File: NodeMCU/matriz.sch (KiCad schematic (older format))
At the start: 16 parts, among them J1 Conn_01x05, Q1 Q_NPN_CBE, Q2 Q_NPN_CBE, Q3 Q_NPN_CBE, SW1 SW_Push_Open, SW2 SW_Push, U3 NodeMCU1.0(ESP-12E)

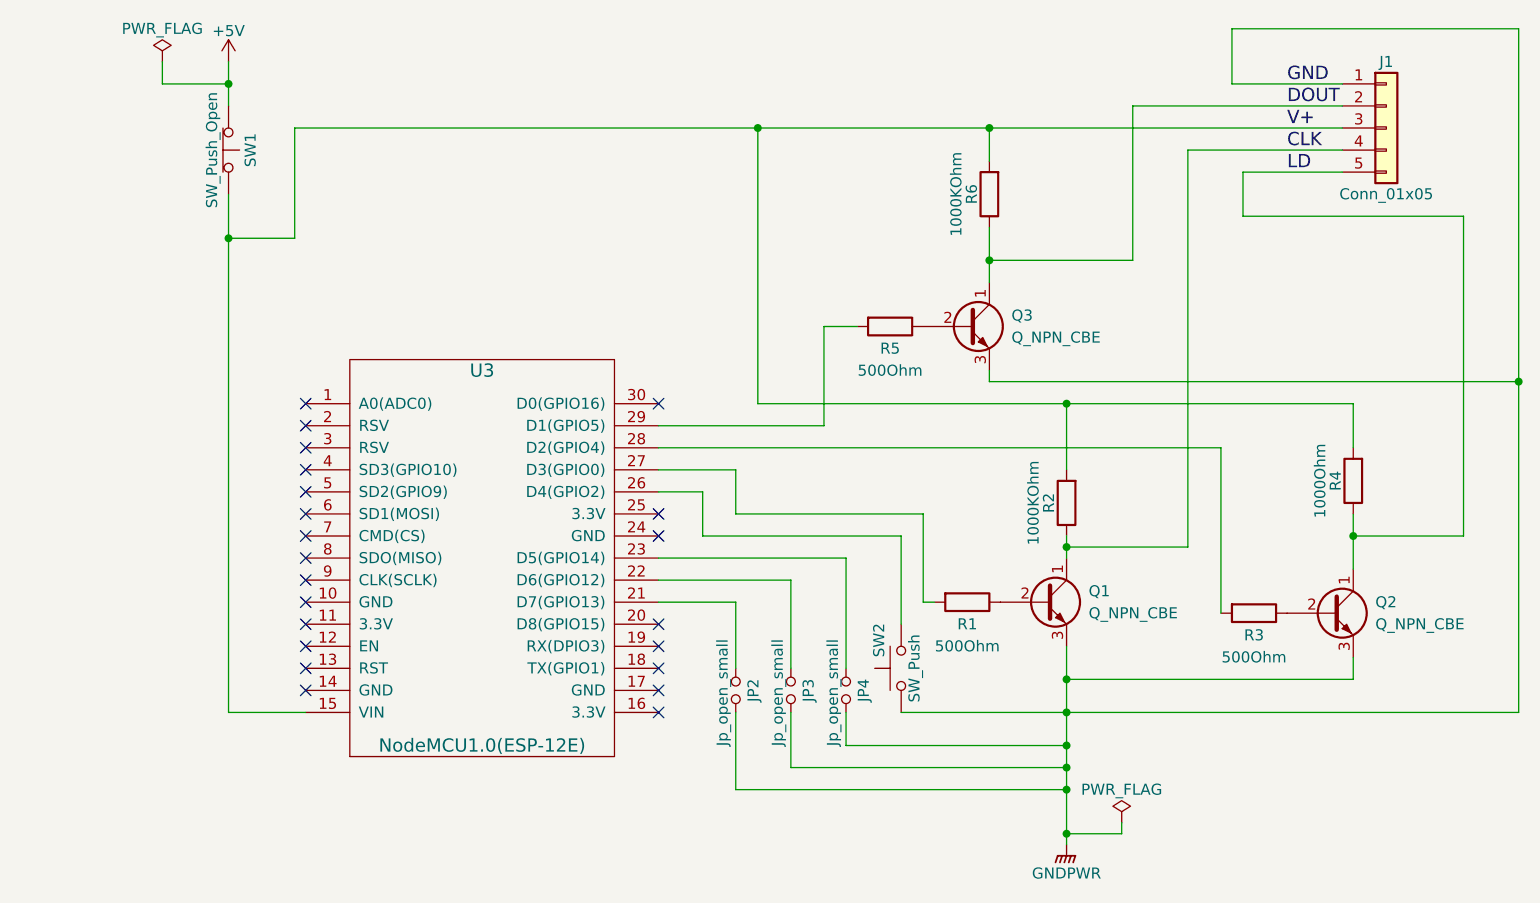
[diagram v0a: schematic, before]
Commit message: Ultimos cambios
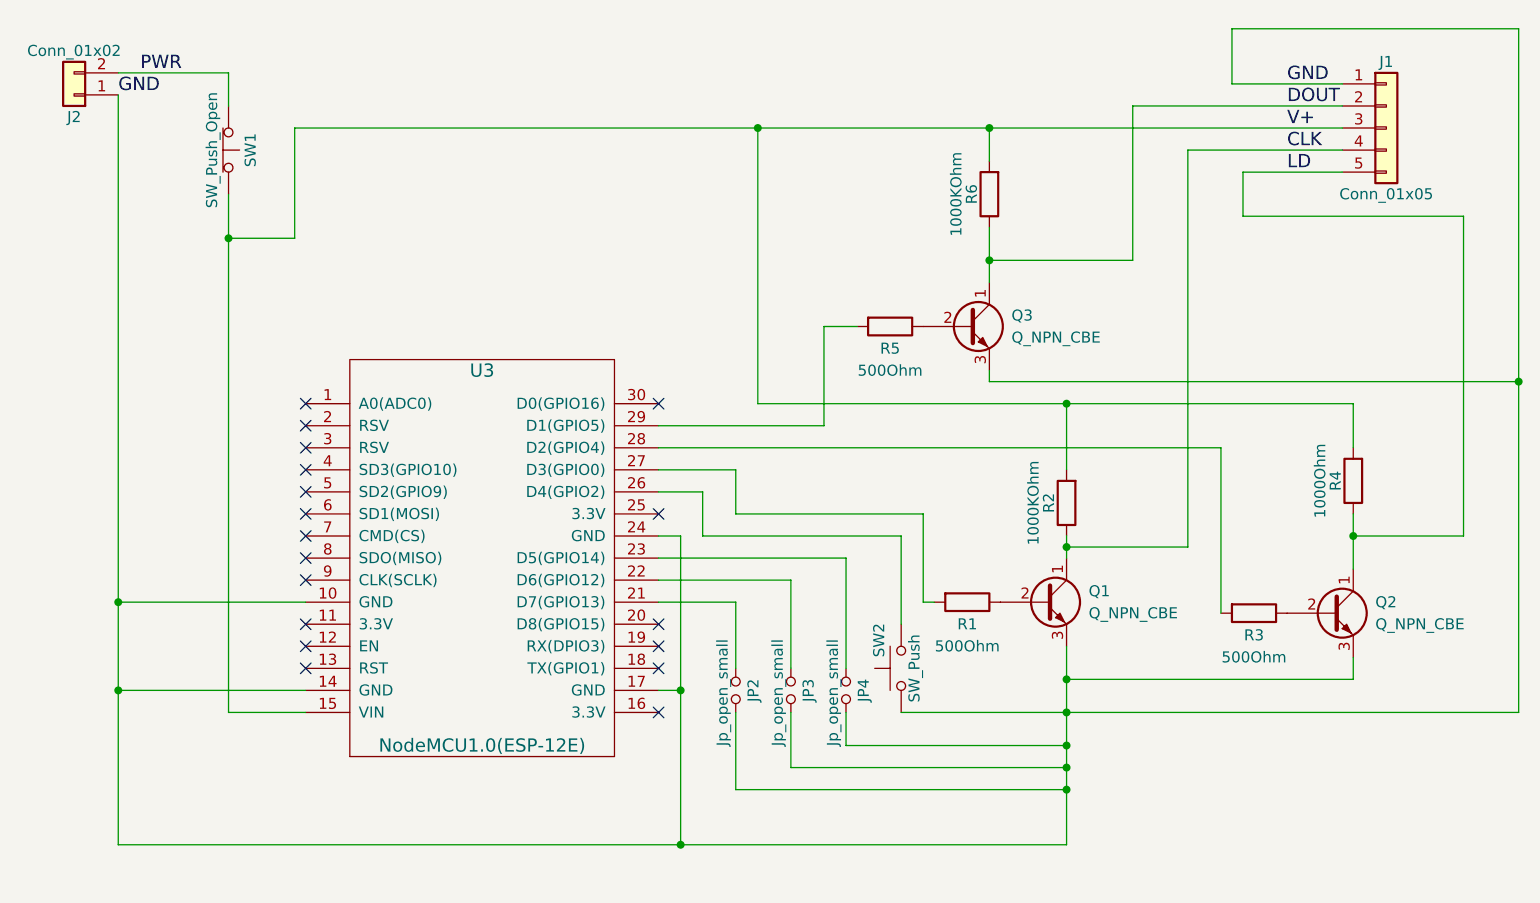
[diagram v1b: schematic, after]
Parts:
- added J2: Conn_01x02, Pin_Headers:Pin_Header_Straight_1x02_Pitch2.54mm, symbol Conn_01x02
- U3: footprint ESP8266:NodeMCU1.0(12-E) -> lib:NodeMCU1.0(12-E)
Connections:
- net GNDPWR is gone; now on net GND: J1.1 (Pin_1), JP2.2, JP3.2, JP4.2, Q1.3 (E), Q2.3 (E), Q3.3 (E), SW2.1
- net GND: now reaches U3.10 (GND)
- net GND: now also U3.14 (GND), U3.17 (GND), U3.24 (GND), J2.1 (Pin_1)
- net +5V renamed PWR
- net PWR: now also J2.2 (Pin_2)
- no-connect marks 22 -> 18
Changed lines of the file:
@@
 F 0 "U3" H 4950 5750 60  0000 C CNN
 F 1 "NodeMCU1.0(ESP-12E)" H 4950 4050 60  0000 C CNN
-F 2 "ESP8266:NodeMCU1.0(12-E)" H 4350 4050 60  0001 C CNN
+F 2 "lib:NodeMCU1.0(12-E)" H 4350 4050 60  0001 C CNN
 F 3 "" H 4350 4050 60  0000 C CNN
 	1    4950 4900
@@
 $EndComp
 NoConn ~ 5750 4700
-NoConn ~ 5750 4800
 NoConn ~ 4150 4200
 NoConn ~ 4150 4300
@@
 NoConn ~ 5750 5300
 NoConn ~ 5750 5400
-NoConn ~ 5750 5500
 NoConn ~ 5750 5600
-NoConn ~ 4150 5500
-NoConn ~ 4150 5100
 NoConn ~ 4150 4900
 $Comp
@@
 $EndComp
 NoConn ~ 5750 4200
-$Comp
-L +5V #PWR01
-U 1 1 5A00823B
-P 3800 2650
-F 0 "#PWR01" H 3800 2500 50  0001 C CNN
-F 1 "+5V" H 3800 2790 50  0000 C CNN
-F 2 "" H 3800 2650 50  0001 C CNN
-F 3 "" H 3800 2650 50  0001 C CNN
-	1    3800 2650
-	1    0    0    -1
-$EndComp
-$Comp
-L PWR_FLAG #FLG02
-U 1 1 5A090401
-P 3500 2650
-F 0 "#FLG02" H 3500 2725 50  0001 C CNN
-F 1 "PWR_FLAG" H 3500 2800 50  0000 C CNN
-F 2 "" H 3500 2650 50  0001 C CNN
-F 3 "" H 3500 2650 50  0001 C CNN
-	1    3500 2650
-	1    0    0    -1
-$EndComp
 NoConn ~ 5750 5200
 Text Label 8600 2750 0    60   ~ 0
@@
 $EndComp
 $Comp
-L PWR_FLAG #FLG03
-U 1 1 5A09C060
-P 7850 6100
-F 0 "#FLG03" H 7850 6175 50  0001 C CNN
-F 1 "PWR_FLAG" H 7850 6250 50  0000 C CNN
-F 2 "" H 7850 6100 50  0001 C CNN
-F 3 "" H 7850 6100 50  0001 C CNN
-	1    7850 6100
-	1    0    0    -1
-$EndComp
-$Comp
 L R R1
 U 1 1 5A048190
@@
 $EndComp
 $Comp
-L GNDPWR #PWR04
-U 1 1 5A09BA2F
-P 7600 6200
-F 0 "#PWR04" H 7600 6000 50  0001 C CNN
-F 1 "GNDPWR" H 7600 6070 50  0000 C CNN
-F 2 "" H 7600 6150 50  0001 C CNN
-F 3 "" H 7600 6150 50  0001 C CNN
-	1    7600 6200
-	1    0    0    -1
-$EndComp
-$Comp
 L R R5
 U 1 1 5A0A44A8
@@
 Connection ~ 7600 5450
 Wire Wire Line
-	7600 5300 7600 6200
-Wire Wire Line
 	8900 5450 7600 5450
 Connection ~ 7600 5750
@@
 Wire Wire Line
 	9400 3350 8400 3350
-Connection ~ 7600 6150
-Wire Wire Line
-	7850 6150 7850 6100
-Wire Wire Line
-	7600 6150 7850 6150
 Wire Wire Line
 	6600 5750 7600 5750
@@
 Wire Wire Line
 	8350 2500 8350 2750
-Connection ~ 3800 2750
-Wire Wire Line
-	3500 2750 3500 2650
-Wire Wire Line
-	3800 2750 3500 2750
 Wire Wire Line
 	6350 5000 6350 5400
@@
 Wire Wire Line
 	7900 2850 8850 2850
-Wire Wire Line
-	3800 2650 3800 2850
+$Comp
+L Conn_01x02 J2
+U 1 1 5A2EF212
+P 3100 2800
+F 0 "J2" H 3100 2900 50  0000 C CNN
+F 1 "Conn_01x02" H 3100 2600 50  0000 C CNN
+F 2 "Pin_Headers:Pin_Header_Straight_1x02_Pitch2.54mm" H 3100 2800 50  0001 C CNN
+F 3 "" H 3100 2800 50  0001 C CNN
+	1    3100 2800
+	-1   0    0    1
+$EndComp
+Wire Wire Line
+	3800 2850 3800 2700
+Wire Wire Line
+	3800 2700 3300 2700
+Wire Wire Line
+	7600 5300 7600 6200
+Wire Wire Line
+	7600 6200 3300 6200
+Wire Wire Line
+	3300 6200 3300 2800
+Text Label 3400 2700 0    60   ~ 0
+PWR
+Text Label 3300 2800 0    60   ~ 0
+GND
+Wire Wire Line
+	4150 5500 3300 5500
+Connection ~ 3300 5500
+Wire Wire Line
+	5750 5500 5850 5500
+Wire Wire Line
+	5850 4800 5850 6200
+Connection ~ 5850 6200
+Wire Wire Line
+	4150 5100 3300 5100
+Connection ~ 3300 5100
+Wire Wire Line
+	5750 4800 5850 4800
+Connection ~ 5850 5500
 $EndSCHEMATC
